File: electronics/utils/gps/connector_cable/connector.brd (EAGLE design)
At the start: 17.4 x 22.9 mm, 2 parts, among them X1 87758-2016

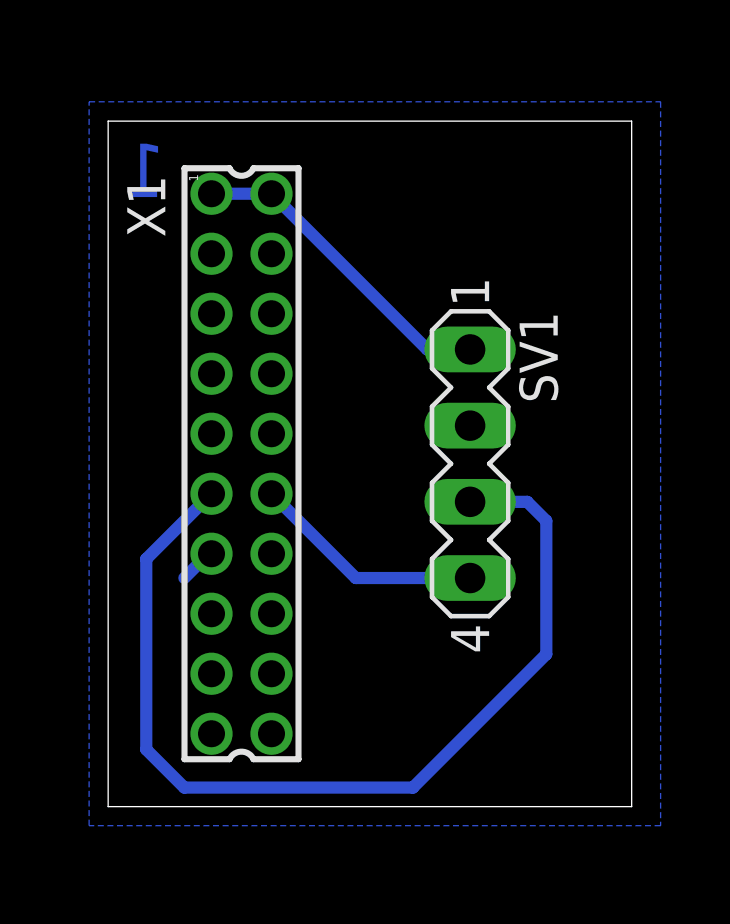
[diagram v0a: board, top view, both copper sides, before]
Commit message: atualizando computador
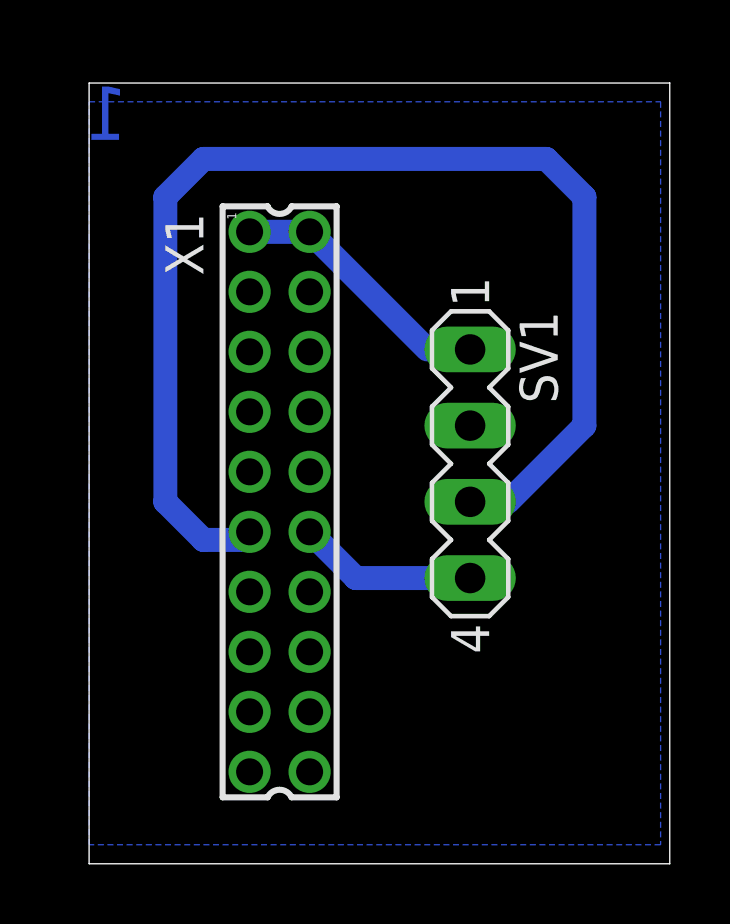
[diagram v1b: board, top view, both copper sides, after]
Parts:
- moved X1 1.80 mm to (7.62, 10.2)
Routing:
- net TX: track 32.4 -> 41.1 mm
- net VCC: track 10.8 -> 8.97 mm
- net RX: track 7.78 -> 5.99 mm
- net GND: track 1.24 -> 0.00 mm
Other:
- board size 17.4 x 22.9 mm -> 19.4 x 26 mm
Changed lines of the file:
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@@
 <board>
 <plain>
-<wire x1="1.905" y1="0" x2="19.355" y2="0" width="0" layer="20"/>
-<wire x1="19.355" y1="0" x2="19.355" y2="22.85" width="0" layer="20"/>
-<wire x1="19.355" y1="22.85" x2="1.905" y2="22.85" width="0" layer="20"/>
-<wire x1="1.905" y1="22.85" x2="1.905" y2="0" width="0" layer="20"/>
-<text x="3.81" y="20.32" size="1.778" layer="16" rot="MR0">1</text>
+<wire x1="1.27" y1="-1.905" x2="20.625" y2="-1.905" width="0" layer="20"/>
+<wire x1="20.625" y1="-1.905" x2="20.625" y2="24.12" width="0" layer="20"/>
+<wire x1="20.625" y1="24.12" x2="1.27" y2="24.12" width="0" layer="20"/>
+<wire x1="1.27" y1="24.12" x2="1.27" y2="-1.905" width="0" layer="20"/>
+<text x="2.54" y="22.225" size="1.778" layer="16" rot="MR0">1</text>
 </plain>
 <attributes>
@@
 <pass name="Default">
 <param name="RoutingGrid" value="50mil"/>
-<param name="tpViaShape" value="round"/>
+<param name="tpViaShape" value="octagon"/>
 <param name="PrefDir.1" value="|"/>
 <param name="PrefDir.2" value="0"/>
@@
 </autorouter>
 <elements>
-<element name="X1" library="con-molex" package="87758-2016" value="87758-2016" x="6.35" y="11.43" rot="R270">
-<attribute name="OC_NEWARK" value="25M5677" x="1.27" y="-11.43" size="1.778" layer="27" rot="R270" display="off"/>
-<attribute name="MPN" value="87758-2016" x="1.27" y="-11.43" size="1.778" layer="27" rot="R270" display="off"/>
-<attribute name="MF" value="" x="1.27" y="-11.43" size="1.778" layer="27" rot="R270" display="off"/>
-<attribute name="OC_FARNELL" value="7472374" x="1.27" y="-11.43" size="1.778" layer="27" rot="R270" display="off"/>
+<element name="X1" library="con-molex" package="87758-2016" value="87758-2016" x="7.62" y="10.16" rot="R270">
+<attribute name="OC_NEWARK" value="25M5677" x="2.54" y="-12.7" size="1.778" layer="27" rot="R270" display="off"/>
+<attribute name="MPN" value="87758-2016" x="2.54" y="-12.7" size="1.778" layer="27" rot="R270" display="off"/>
+<attribute name="MF" value="" x="2.54" y="-12.7" size="1.778" layer="27" rot="R270" display="off"/>
+<attribute name="OC_FARNELL" value="7472374" x="2.54" y="-12.7" size="1.778" layer="27" rot="R270" display="off"/>
 </element>
 <element name="SV1" library="con-lstb" package="MA04-1" value="" x="13.97" y="11.43" rot="R270">
@@
 <contactref element="SV1" pad="1"/>
 <wire x1="13.97" y1="15.24" x2="12.54" y2="15.24" width="0.4064" layer="16"/>
-<wire x1="12.54" y1="15.24" x2="7.35" y2="20.43" width="0.4064" layer="16"/>
-<wire x1="7.35" y1="20.43" x2="5.35" y2="20.43" width="0.4064" layer="16"/>
+<wire x1="12.54" y1="15.24" x2="8.62" y2="19.16" width="0.8001" layer="16"/>
+<wire x1="8.62" y1="19.16" x2="6.62" y2="19.16" width="0.8001" layer="16"/>
 </signal>
 <signal name="GND">
@@
 <contactref element="X1" pad="18"/>
 <contactref element="SV1" pad="2"/>
-<polygon width="0.4064" layer="16">
-<vertex x="1.27" y="-0.635"/>
+<polygon width="0.4064" layer="16" isolate="0.4064">
+<vertex x="1.27" y="-1.27"/>
 <vertex x="1.27" y="23.495"/>
 <vertex x="20.32" y="23.495"/>
-<vertex x="20.32" y="-0.635"/>
+<vertex x="20.32" y="-1.27"/>
 </polygon>
-<wire x1="5.35" y1="8.43" x2="5.255" y2="8.43" width="0.4064" layer="16"/>
-<wire x1="5.255" y1="8.43" x2="4.445" y2="7.62" width="0.4064" layer="16"/>
+<wire x1="6.62" y1="7.16" x2="8.62" y2="11.16" width="0" layer="19" extent="1-1"/>
 </signal>
 <signal name="TX">
 <contactref element="X1" pad="11"/>
 <contactref element="SV1" pad="3"/>
-<wire x1="13.97" y1="10.16" x2="15.875" y2="10.16" width="0.4064" layer="16"/>
-<wire x1="15.875" y1="10.16" x2="16.51" y2="9.525" width="0.4064" layer="16"/>
-<wire x1="16.51" y1="9.525" x2="16.51" y2="5.08" width="0.4064" layer="16"/>
-<wire x1="16.51" y1="5.08" x2="12.065" y2="0.635" width="0.4064" layer="16"/>
-<wire x1="12.065" y1="0.635" x2="4.445" y2="0.635" width="0.4064" layer="16"/>
-<wire x1="4.445" y1="0.635" x2="3.175" y2="1.905" width="0.4064" layer="16"/>
-<wire x1="3.175" y1="1.905" x2="3.175" y2="8.255" width="0.4064" layer="16"/>
-<wire x1="3.175" y1="8.255" x2="5.35" y2="10.43" width="0.4064" layer="16"/>
+<wire x1="13.97" y1="10.16" x2="15.24" y2="10.16" width="0.4064" layer="16"/>
+<wire x1="15.24" y1="10.16" x2="17.78" y2="12.7" width="0.8001" layer="16"/>
+<wire x1="17.78" y1="12.7" x2="17.78" y2="20.32" width="0.8001" layer="16"/>
+<wire x1="17.78" y1="20.32" x2="16.51" y2="21.59" width="0.8001" layer="16"/>
+<wire x1="16.51" y1="21.59" x2="5.08" y2="21.59" width="0.8001" layer="16"/>
+<wire x1="5.08" y1="21.59" x2="3.81" y2="20.32" width="0.8001" layer="16"/>
+<wire x1="3.81" y1="20.32" x2="3.81" y2="10.16" width="0.8001" layer="16"/>
+<wire x1="3.81" y1="10.16" x2="5.08" y2="8.89" width="0.8001" layer="16"/>
+<wire x1="5.08" y1="8.89" x2="6.35" y2="8.89" width="0.8001" layer="16"/>
+<wire x1="6.35" y1="8.89" x2="6.62" y2="9.16" width="0.4064" layer="16"/>
 </signal>
 <signal name="RX">
 <contactref element="X1" pad="12"/>
 <contactref element="SV1" pad="4"/>
-<wire x1="13.97" y1="7.62" x2="10.16" y2="7.62" width="0.4064" layer="16"/>
-<wire x1="10.16" y1="7.62" x2="7.35" y2="10.43" width="0.4064" layer="16"/>
+<wire x1="13.97" y1="7.62" x2="10.16" y2="7.62" width="0.8001" layer="16"/>
+<wire x1="10.16" y1="7.62" x2="8.62" y2="9.16" width="0.8001" layer="16"/>
 </signal>
 </signals>
